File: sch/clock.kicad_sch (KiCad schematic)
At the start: 7 parts, among them U2 74AHC74

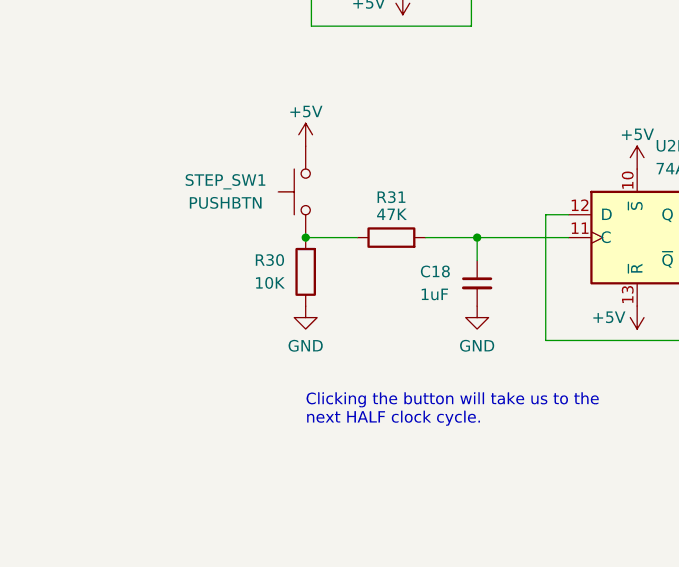
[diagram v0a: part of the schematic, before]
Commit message: Clearances
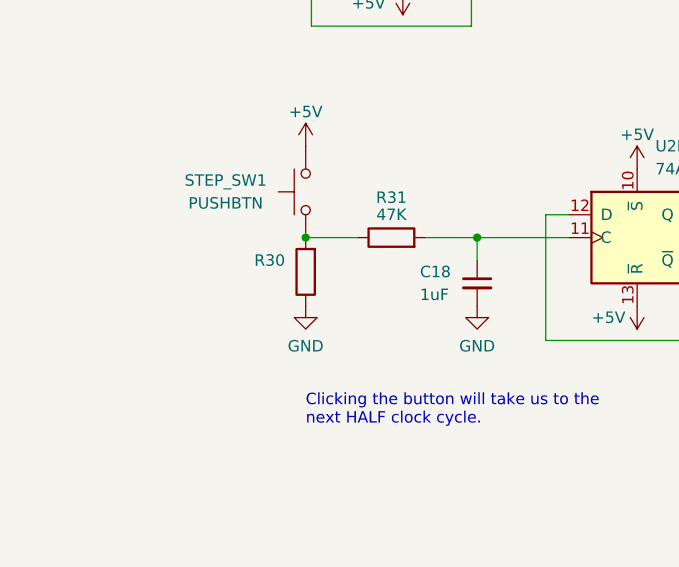
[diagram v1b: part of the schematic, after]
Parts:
- R30: value 10K -> (none)
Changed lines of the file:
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@@
       (effects (font (size 1.27 1.27)) (justify right))
     )
-    (property "Value" "10K" (id 1) (at 57.785 88.265 0)
+    (property "Value" "" (id 1) (at 57.785 88.265 0)
       (effects (font (size 1.27 1.27)) (justify right))
     )
